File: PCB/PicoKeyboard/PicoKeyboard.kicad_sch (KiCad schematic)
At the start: 5 parts, among them J1 USB_C_Receptacle_USB2.0_14P, J2 Conn_01x04_Socket, U1 Raspberry_Pi_Pico

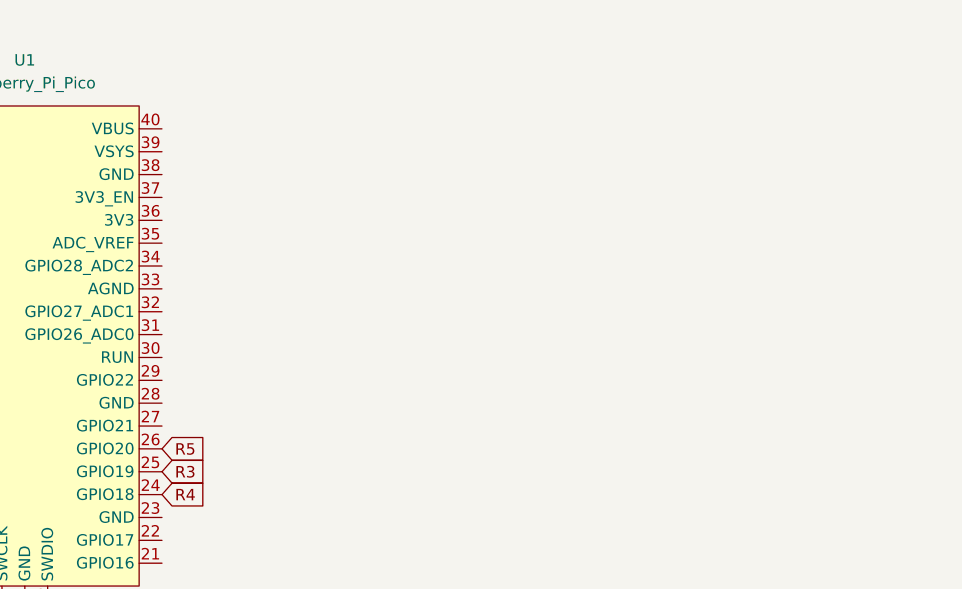
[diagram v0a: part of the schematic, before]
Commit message: Add screen header pin
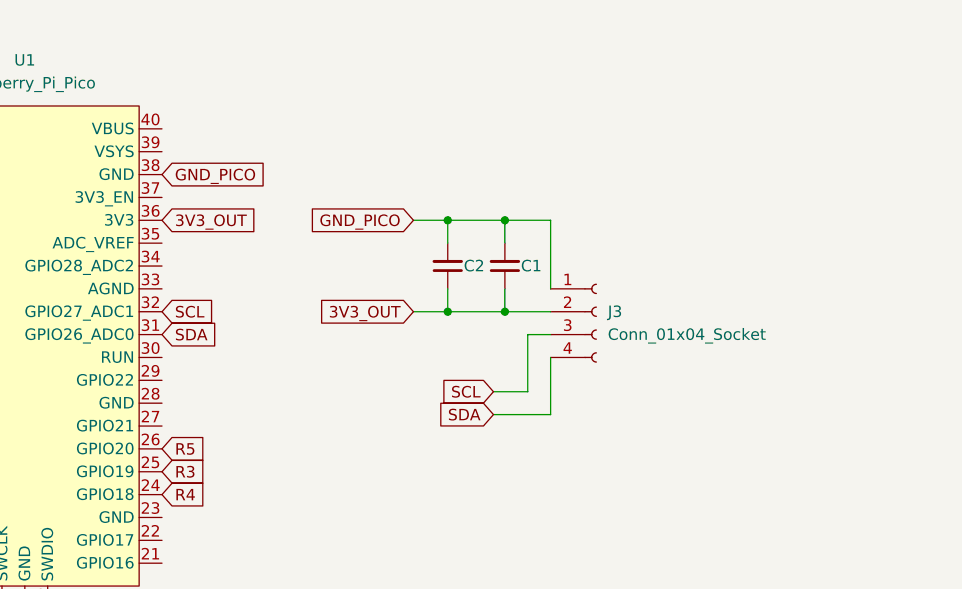
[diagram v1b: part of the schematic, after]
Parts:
- added C1, C2: C_Small, Capacitor_SMD:C_0201_0603Metric_Pad0.64x0.40mm_HandSolder, symbol Device:C_Small
- added J3: Conn_01x04_Socket, Connector_PinSocket_2.54mm:PinSocket_1x04_P2.54mm_Vertical, symbol Connector:Conn_01x04_Socket
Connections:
- net SDA: now reaches U1.31 (GPIO26_ADC0)
- net SDA: now also J3.4 (Pin_4)
- net SCL: now reaches U1.32 (GPIO27_ADC1)
- net SCL: now also J3.3 (Pin_3)
- net 3V3_OUT: now reaches U1.36 (3V3)
- net 3V3_OUT: now also C1.1, C2.1, J3.2 (Pin_2)
- net GND_PICO: now reaches U1.38 (GND)
- net GND_PICO: now also C1.2, C2.2, J3.1 (Pin_1)

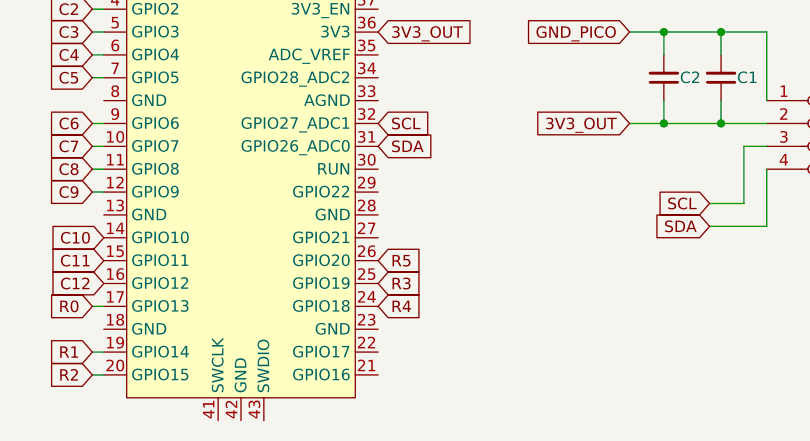
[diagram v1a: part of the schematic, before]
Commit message: Update PCB
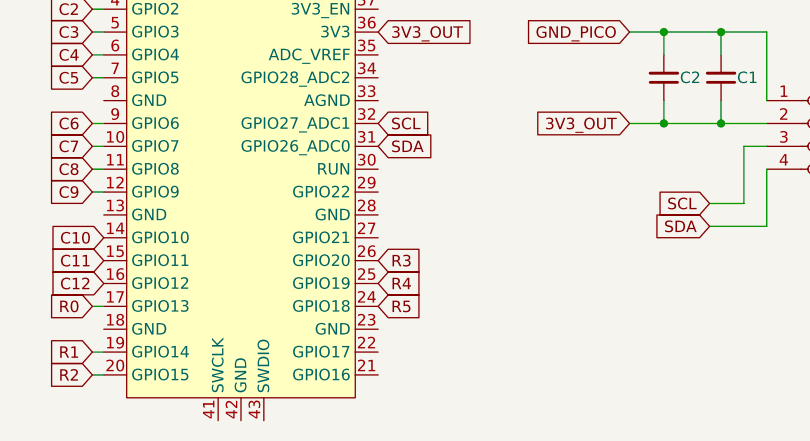
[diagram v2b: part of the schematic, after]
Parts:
- R1, R2: footprint Resistor_SMD:R_0201_0603Metric_Pad0.64x0.40mm_HandSolder -> Resistor_SMD:R_0201_0603Metric
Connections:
- net R3: now also U1.26 (GPIO20); no longer U1.25 (GPIO19)
- net R4: now also U1.25 (GPIO19); no longer U1.24 (GPIO18)
- net R5: now also U1.24 (GPIO18); no longer U1.26 (GPIO20)
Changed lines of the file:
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@@
 	(global_label "R4"
 		(shape input)
-		(at 87.63 139.7 0)
+		(at 87.63 137.16 0)
 		(fields_autoplaced yes)
 		(effects
@@
 		)
 		(property "Intersheetrefs" "${INTERSHEET_REFS}"
-			(at 93.0947 139.7 0)
+			(at 93.0947 137.16 0)
 			(effects
 				(font
@@
 	(global_label "R5"
 		(shape input)
-		(at 87.63 134.62 0)
+		(at 87.63 139.7 0)
 		(fields_autoplaced yes)
 		(effects
@@
 		)
 		(property "Intersheetrefs" "${INTERSHEET_REFS}"
-			(at 93.0947 134.62 0)
+			(at 93.0947 139.7 0)
 			(effects
 				(font
@@
 	(global_label "R3"
 		(shape input)
-		(at 87.63 137.16 0)
+		(at 87.63 134.62 0)
 		(fields_autoplaced yes)
 		(effects
@@
 		)
 		(property "Intersheetrefs" "${INTERSHEET_REFS}"
-			(at 93.0947 137.16 0)
+			(at 93.0947 134.62 0)
 			(effects
 				(font
@@
 			)
 		)
-		(property "Footprint" "Resistor_SMD:R_0201_0603Metric_Pad0.64x0.40mm_HandSolder"
+		(property "Footprint" "Resistor_SMD:R_0201_0603Metric"
 			(at 69.85 44.958 0)
 			(effects
@@
 			)
 		)
-		(property "Footprint" "Resistor_SMD:R_0201_0603Metric_Pad0.64x0.40mm_HandSolder"
+		(property "Footprint" "Resistor_SMD:R_0201_0603Metric"
 			(at 69.85 47.498 0)
 			(effects

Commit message: Update PCB
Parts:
- C1: value C_Small -> 100nF
- C2: value C_Small -> 1uF
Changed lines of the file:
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@@
 			)
 		)
-		(property "Value" "C_Small"
+		(property "Value" "1uF"
 			(at 121.92 115.5635 0)
 			(effects
@@
 			)
 		)
-		(property "Value" "C_Small"
+		(property "Value" "100nF"
 			(at 128.27 115.5635 0)
 			(effects

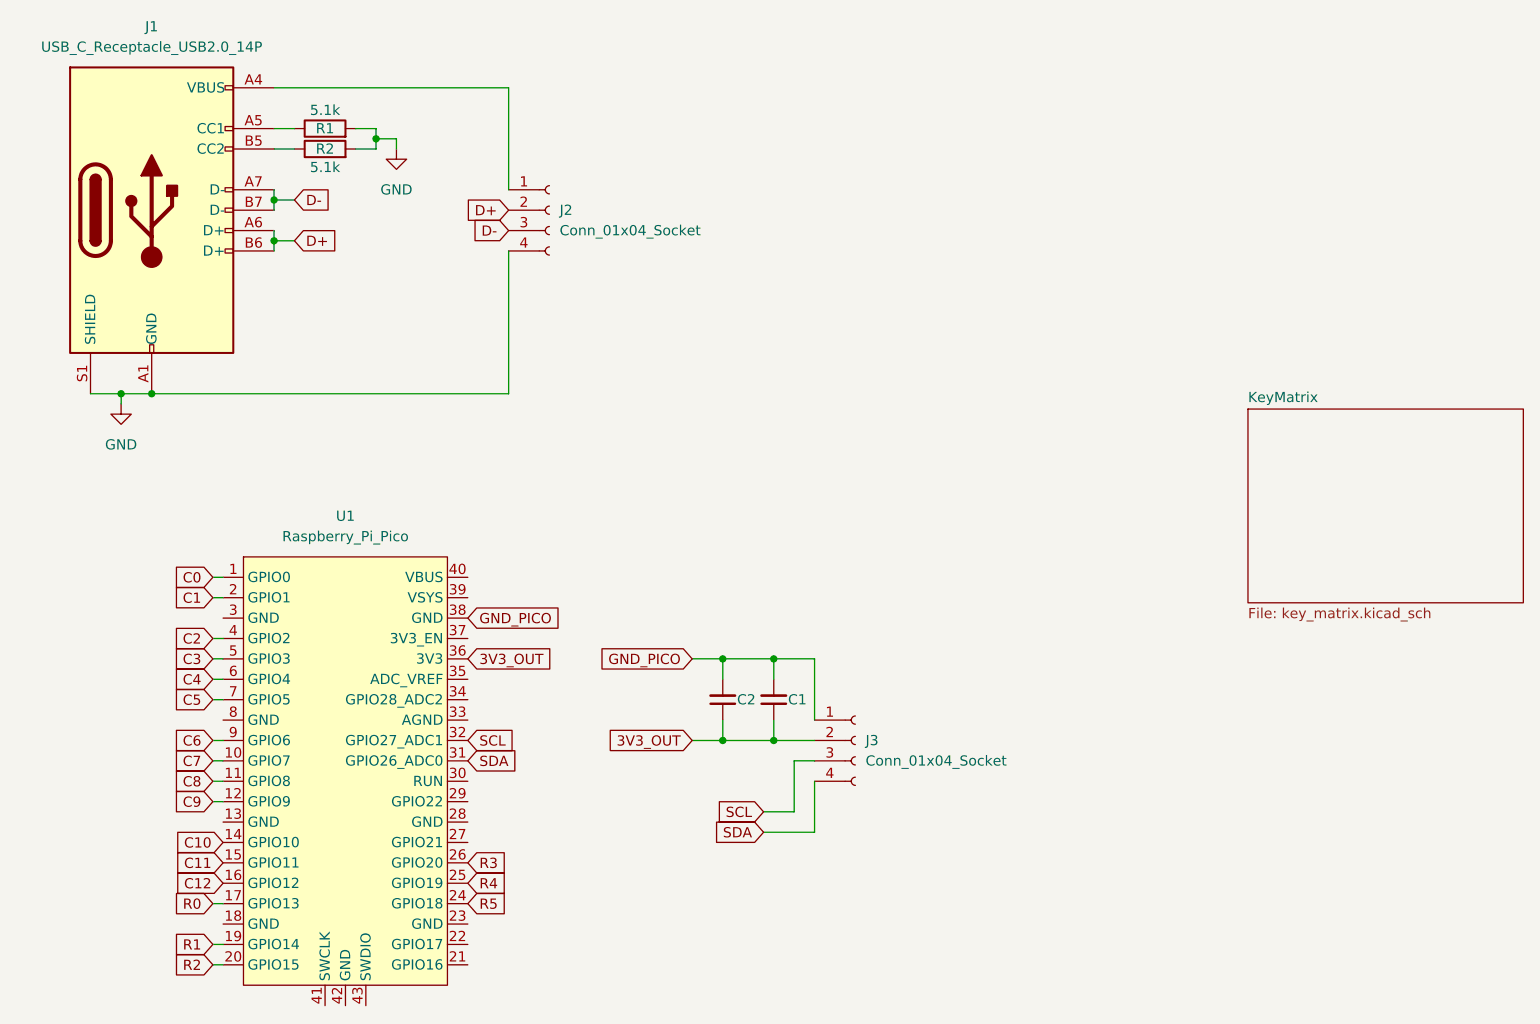
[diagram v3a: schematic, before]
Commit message: Update PCB
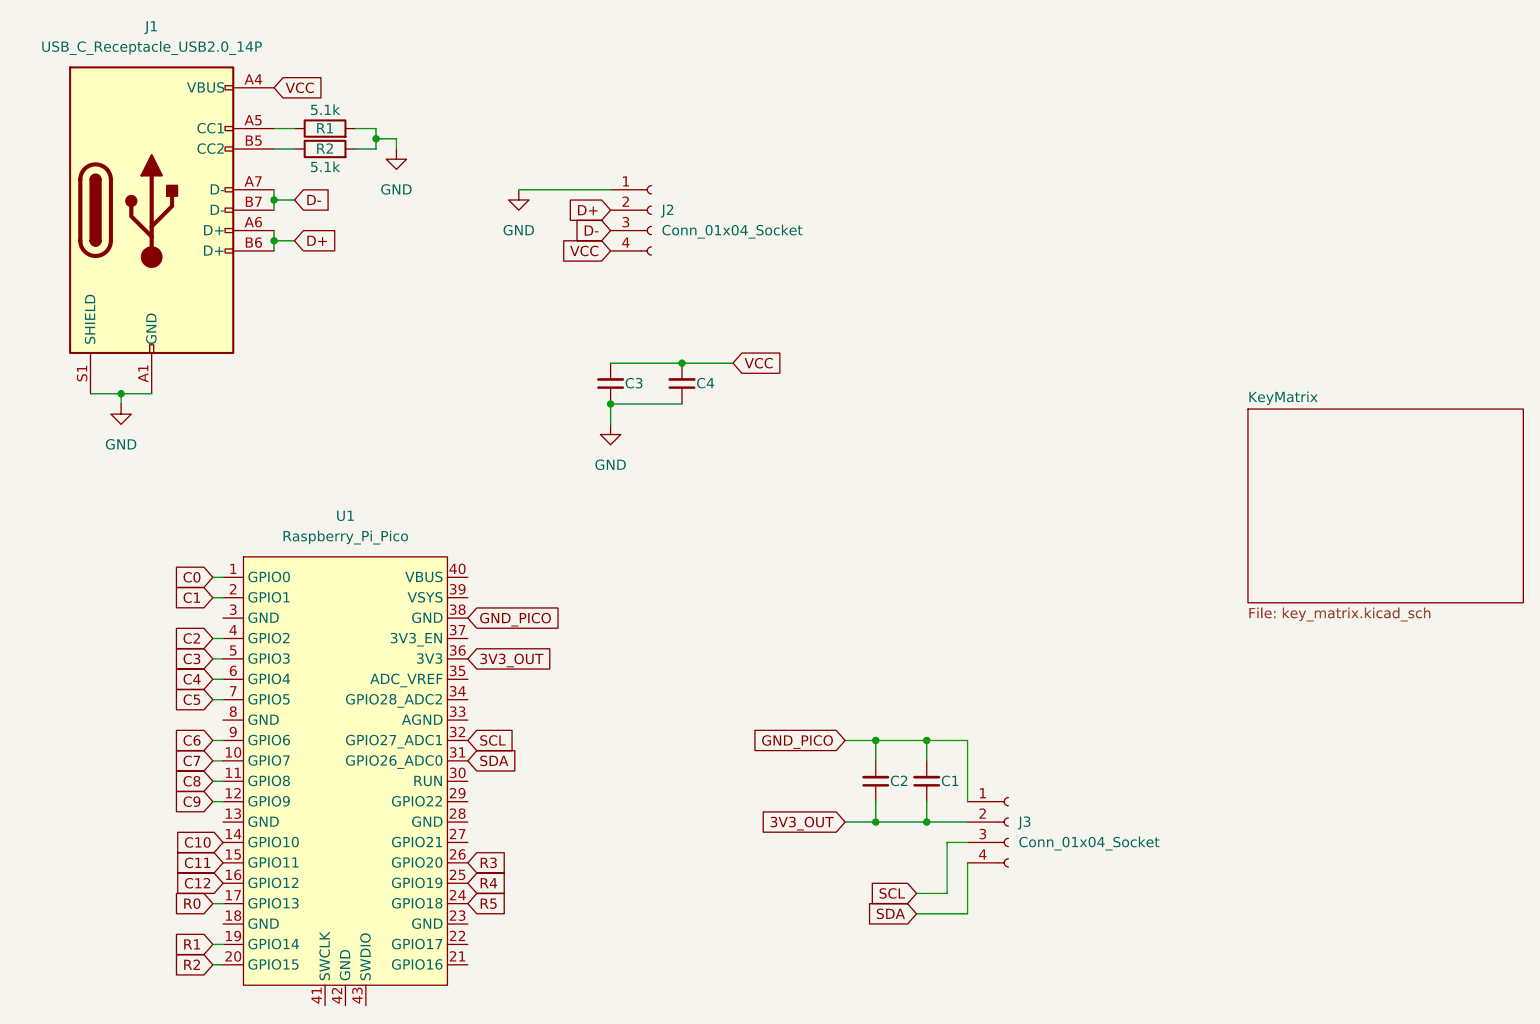
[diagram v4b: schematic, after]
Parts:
- added C3: 1uF, Capacitor_SMD:C_0201_0603Metric_Pad0.64x0.40mm_HandSolder, symbol Device:C_Small
- added C4: 100nF, Capacitor_SMD:C_0201_0603Metric_Pad0.64x0.40mm_HandSolder, symbol Device:C_Small
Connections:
- net GND: now also J2.1 (Pin_1), C3.1, C4.1; no longer J2.4 (Pin_4)
- net VCC: now reaches J1.A4 (VBUS), J1.A9 (VBUS), J1.B4 (VBUS), J1.B9 (VBUS)
- net VCC: now also J2.4 (Pin_4), C3.2, C4.2; no longer J2.1 (Pin_1)
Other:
- moved on the sheet: C1, C2, J2, J3

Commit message: Update PCB
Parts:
- J1: footprint Connector_USB:USB_C_Receptacle_GCT_USB4085 -> Connector_USB:USB_C_Receptacle_GCT_USB4110
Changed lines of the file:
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@@
 			)
 		)
-		(property "Footprint" "Connector_USB:USB_C_Receptacle_GCT_USB4085"
+		(property "Footprint" "Connector_USB:USB_C_Receptacle_GCT_USB4110"
 			(at 52.07 53.34 0)
 			(effects

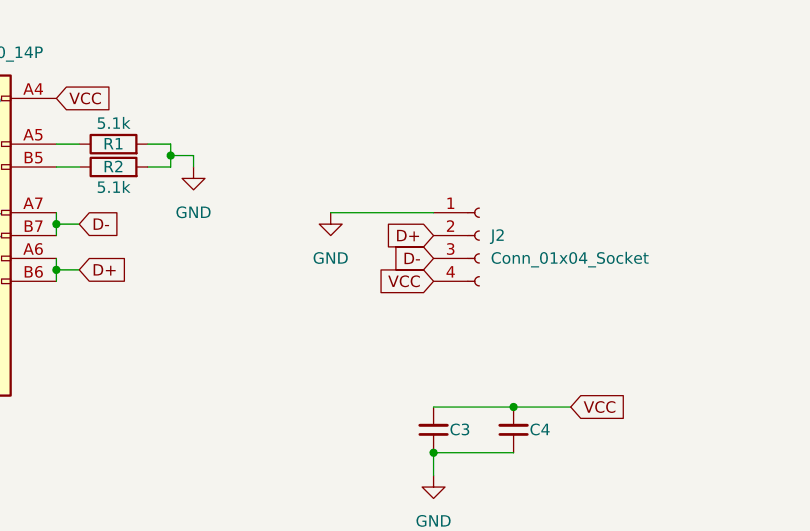
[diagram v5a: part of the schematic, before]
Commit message: Update design
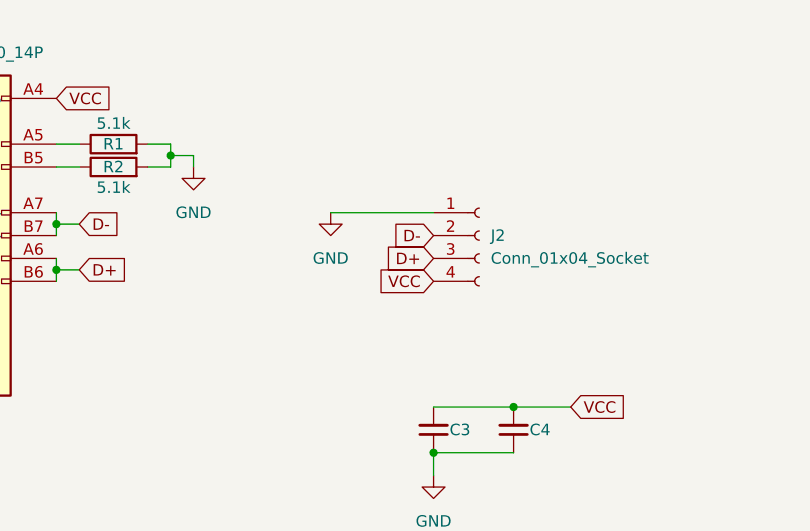
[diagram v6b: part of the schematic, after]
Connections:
- net D+: now also J2.3 (Pin_3); no longer J2.2 (Pin_2)
- net D-: now also J2.2 (Pin_2); no longer J2.3 (Pin_3)
